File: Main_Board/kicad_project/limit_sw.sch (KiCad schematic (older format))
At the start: 70 parts

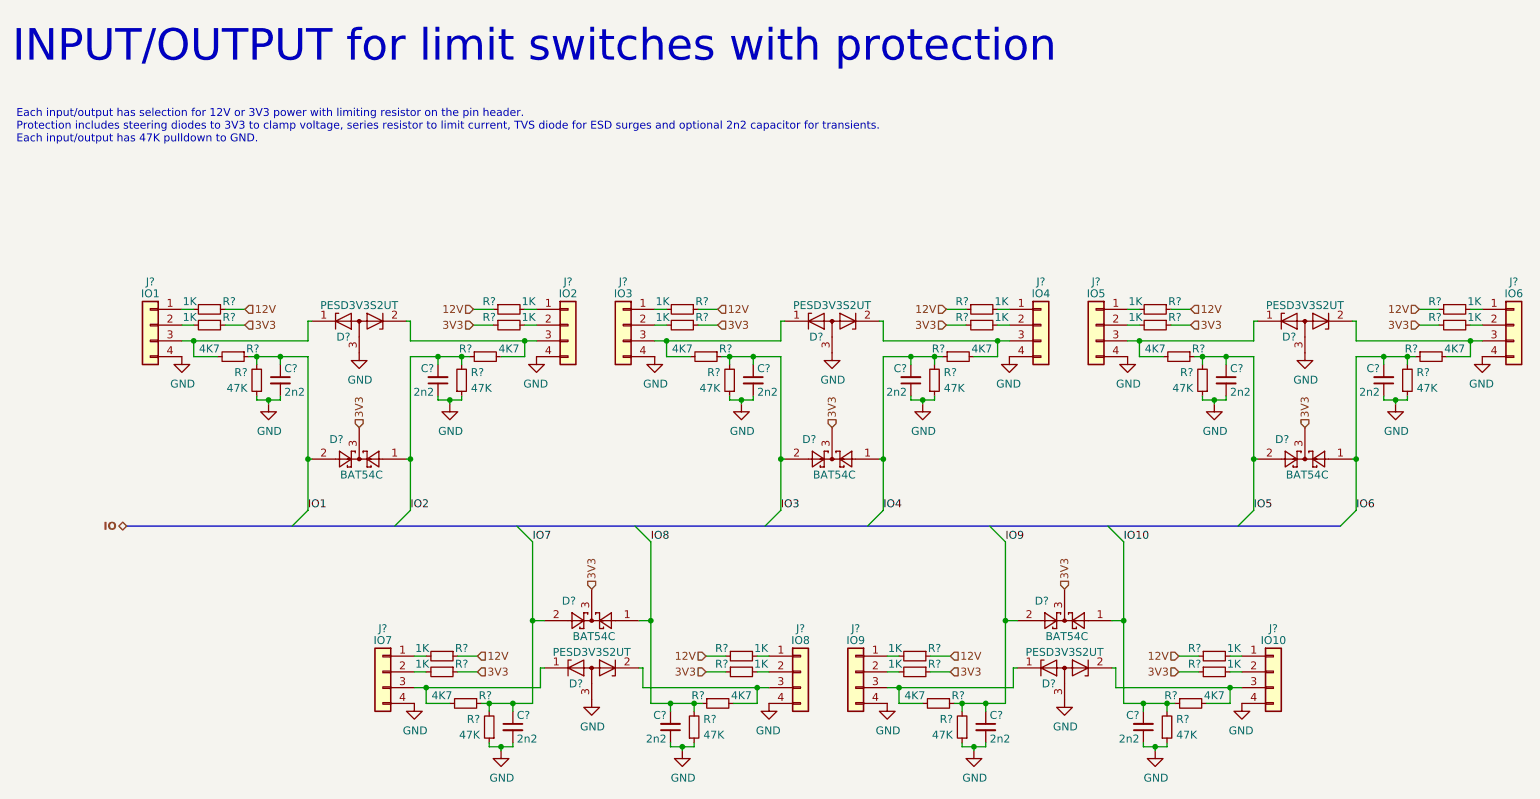
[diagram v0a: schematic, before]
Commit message: progress?
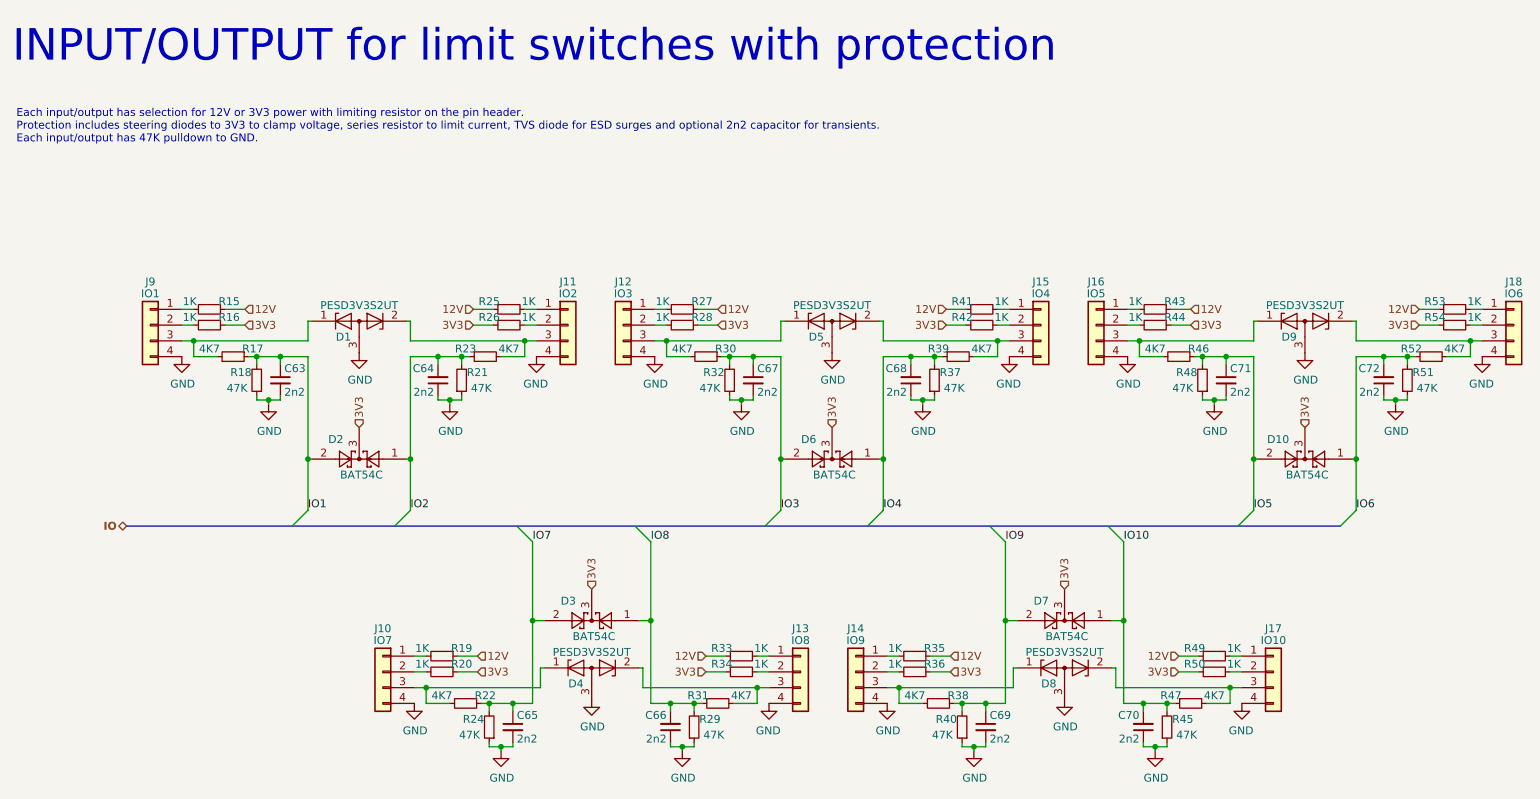
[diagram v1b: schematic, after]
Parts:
- gave numbers to parts that had none: 70

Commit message: progress on MCU pinout
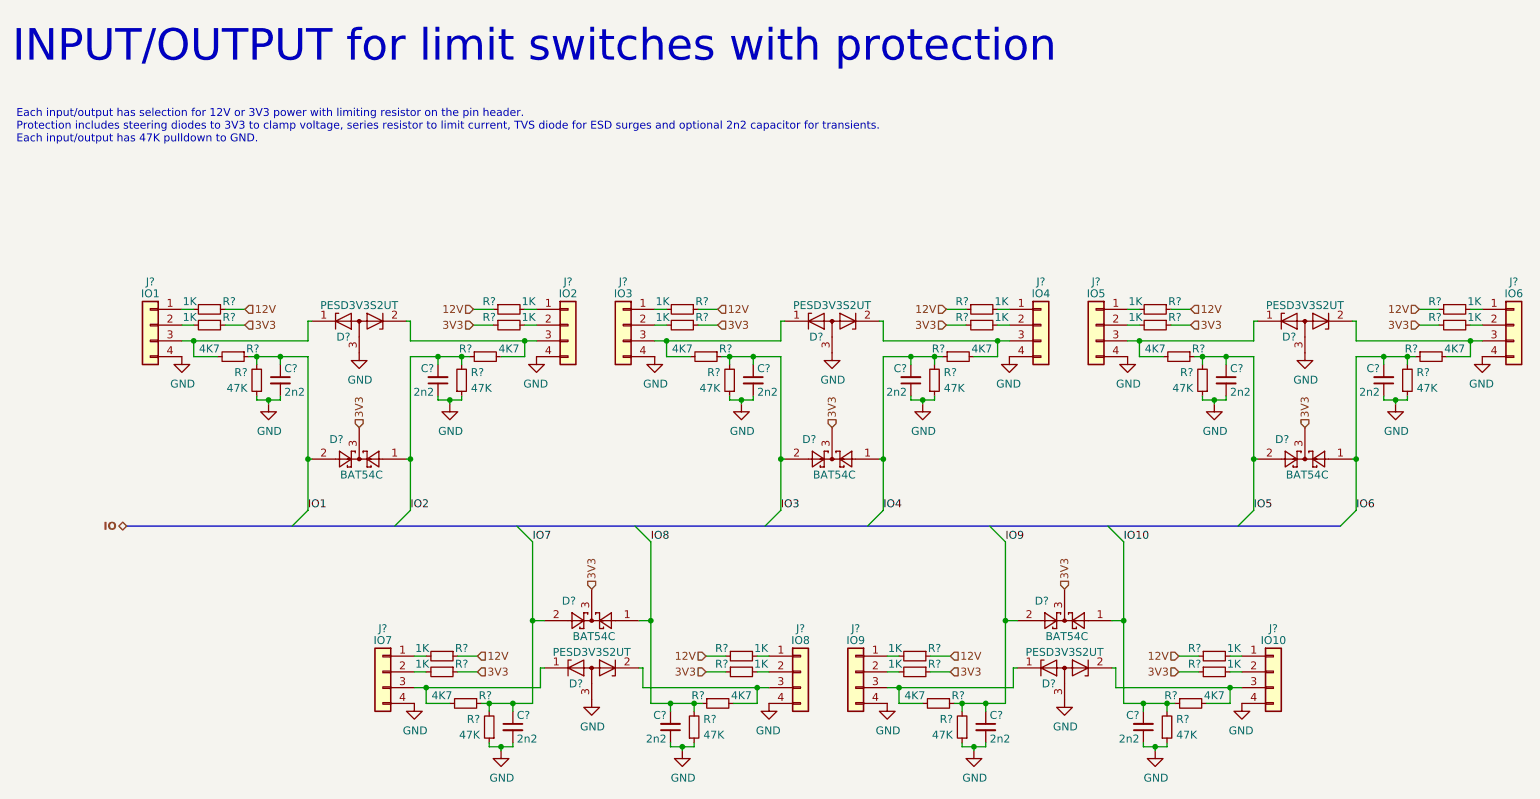
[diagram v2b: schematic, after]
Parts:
- renumbered C63 to C?, C64 to C?, C68 to C?, C67 to C?, C71 to C?, C72 to C?, C66 to C?, C65 to C?, C70 to C?, C69 to C?, D2 to D?, D1 to D?, D6 to D?, D5 to D?, D9 to D?, D10 to D?, D4 to D?, D3 to D?, D8 to D?, D7 to D?, J9 to J?, J11 to J?, J12 to J?, J15 to J?, J18 to J?, J16 to J?, J10 to J?, J13 to J?, J14 to J?, J17 to J?, R15 to R?, R16 to R?, R17 to R?, R25 to R?, R26 to R?, R23 to R?, R18 to R?, R21 to R?, R27 to R?, R28 to R?, R41 to R?, R42 to R?, R39 to R?, R37 to R?, R32 to R?, R30 to R?, R46 to R?, R48 to R?, R51 to R?, R52 to R?, R54 to R?, R53 to R?, R44 to R?, R43 to R?, R19 to R?, R20 to R?, R33 to R?, R34 to R?, R31 to R?, R29 to R?, R24 to R?, R22 to R?, R35 to R?, R36 to R?, R49 to R?, R50 to R?, R47 to R?, R45 to R?, R40 to R?, R38 to R?
